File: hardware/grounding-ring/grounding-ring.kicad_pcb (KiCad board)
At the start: 2 copper layers, 28 x 38.2 mm, 1 part, among them P1 CONN_01X02

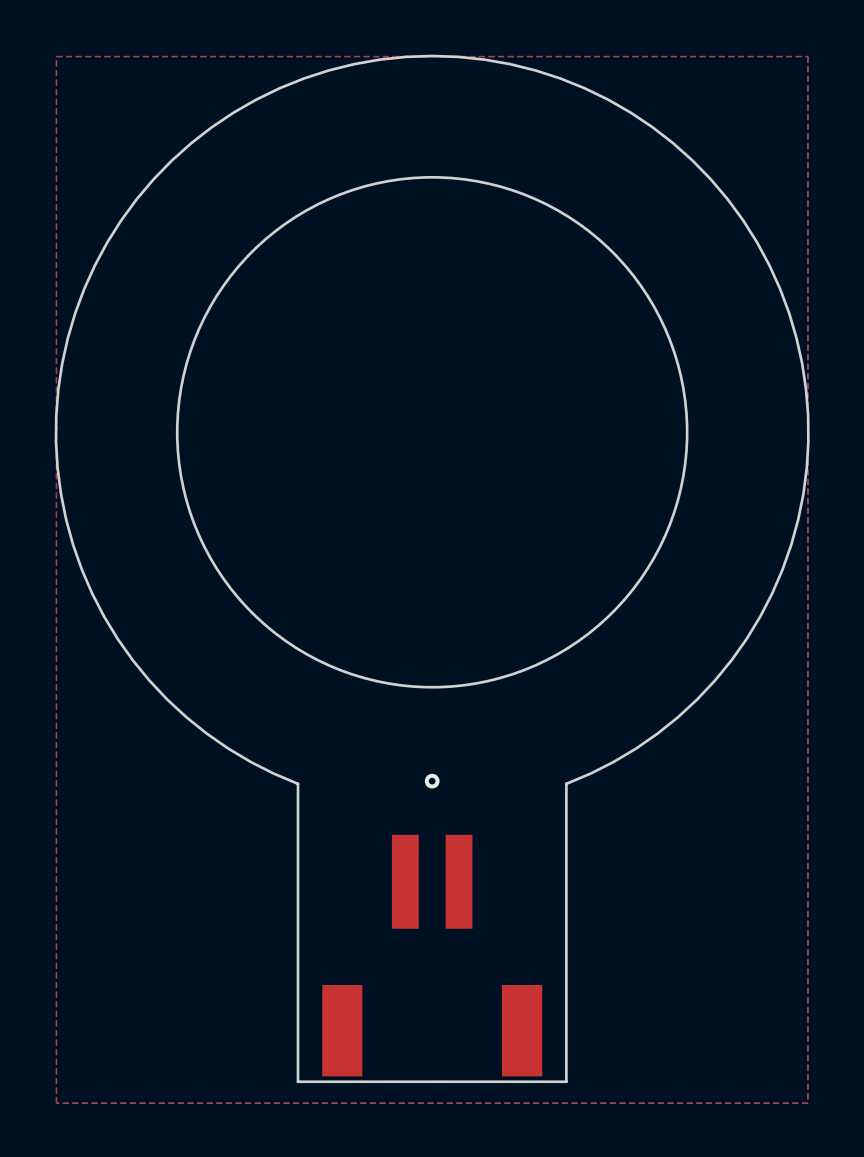
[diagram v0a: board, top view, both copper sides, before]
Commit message: grounding ring prototype
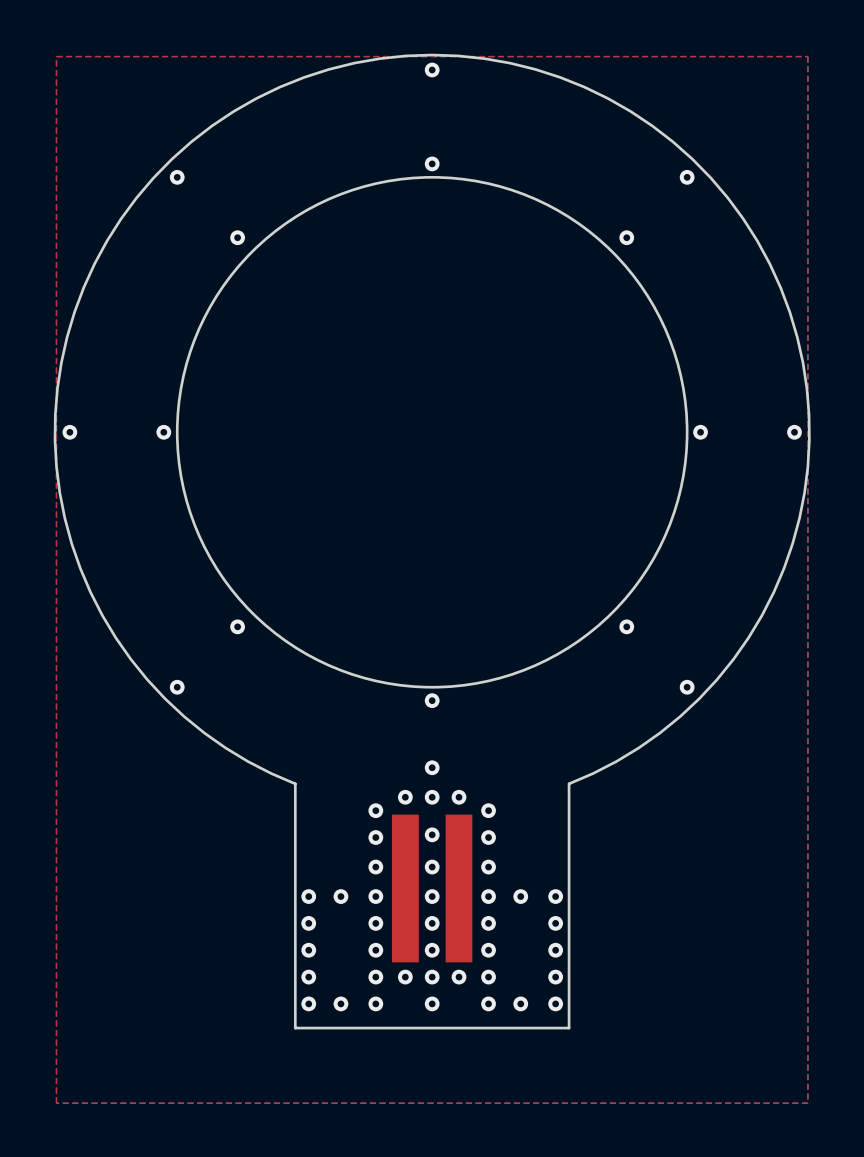
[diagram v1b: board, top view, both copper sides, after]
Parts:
- P1: footprint kicad-libraries:JST-PH-2 -> kicad-libraries:JST-PH-2-SMD
- moved P1 7.00 mm to (150.0, 117.0), turned to 180 degrees
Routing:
- net GND: vias 1 -> 58
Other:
- board size 28 x 38.2 mm -> 28.1 x 36.3 mm
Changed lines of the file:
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@@
     (thickness 1.6)
     (drawings 8)
-    (tracks 1)
+    (tracks 58)
     (zones 0)
     (modules 1)
@@
       (drillshape 0)
       (scaleselection 1)
-      (outputdirectory "../../../Schreibtisch/proto/breakout_V2/"))
+      (outputdirectory "../../../../Schreibtisch/proto/grounding-ring/"))
   )
   (net 0 "")
@@
     (add_net GND)
   )
-  (module kicad-libraries:JST-PH-2 (layer F.Cu)
-    (at 150 124)
-    (fp_text reference P1 (at 0 0) (layer F.Fab)
-      (effects (font (size 0.3 0.3) (thickness 0.075)))
+  (module kicad-libraries:JST-PH-2-SMD (layer F.Cu)
+    (at 150 117 180)
+    (fp_text reference P1 (at 0.09 -3.53) (layer F.Fab)
+      (effects (font (size 0.8 0.8) (thickness 0.15)))
     )
-    (fp_text value CONN_01X02 (at 0 0) (layer F.Fab)
-      (effects (font (size 0.3 0.3) (thickness 0.075)))
+    (fp_text value CONN_01X02 (at 0.48 -0.73) (layer F.Fab)
+      (effects (font (size 0.8 0.8) (thickness 0.15)))
     )
-    (fp_line (start -2.7 0) (end -2.1 -1.2) (layer F.Fab) (width 0.381))
-    (fp_line (start -2.1 -1.2) (end -1.6 0) (layer F.Fab) (width 0.381))
-    (fp_line (start 3.9 0) (end -3.9 0) (layer F.Fab) (width 0.381))
-    (fp_line (start -3.9 0) (end -3.9 -6) (layer F.Fab) (width 0.381))
-    (fp_line (start -3.9 -6) (end 3.9 -6) (layer F.Fab) (width 0.381))
-    (fp_line (start 3.9 -6) (end 3.9 0) (layer F.Fab) (width 0.381))
-    (pad 2 smd rect (at 1 -7.25) (size 1 3.5) (layers F.Cu F.Paste F.Mask)
+    (fp_line (start -3.975 -4.75) (end 3.975 -4.75) (layer F.Fab) (width 0.2))
+    (fp_line (start 3.975 -4.75) (end 3.975 0.25) (layer F.Fab) (width 0.2))
+    (fp_line (start 3.975 0.25) (end -3.975 0.25) (layer F.Fab) (width 0.2))
+    (fp_line (start -3.975 0.25) (end -3.975 -4.75) (layer F.Fab) (width 0.2))
+    (pad "" smd rect (at 3.4 -2.25 180) (size 1.6 3) (layers F.Paste F.Mask))
+    (pad "" smd rect (at -3.4 -2.25 180) (size 1.6 3) (layers F.Paste F.Mask))
+    (pad 2 smd rect (at 1 0 180) (size 1 5.5) (layers F.Cu F.Paste F.Mask)
       (net 1 GND))
-    (pad 1 smd rect (at -1 -7.25) (size 1 3.5) (layers F.Cu F.Paste F.Mask)
+    (pad 1 smd rect (at -1 0 180) (size 1 5.5) (layers F.Cu F.Paste F.Mask)
       (net 1 GND))
-    (pad EP smd rect (at 3.35 -1.7) (size 1.5 3.4) (layers F.Cu F.Paste F.Mask))
-    (pad EP smd rect (at -3.35 -1.7) (size 1.5 3.4) (layers F.Cu F.Paste F.Mask))
+    (model "../3d/Connectors/B2B-PH-SM4-TB(LF)(SN).wrl"
+      (at (xyz 0 0 0))
+      (scale (xyz 1 1 1))
+      (rotate (xyz 0 0 0))
+    )
   )
   (gr_poly (pts (xy 164 113) (xy 136 113) (xy 136 86) (xy 164 86)) (layer B.Mask) (width 0.1))
   (gr_poly (pts (xy 164 113) (xy 136 113) (xy 136 86) (xy 164 86)) (layer F.Mask) (width 0.1))
-  (gr_arc (start 150 100) (end 154.999999 113.099999) (angle -318.2183505) (layer Edge.Cuts) (width 0.1))
-  (gr_line (start 145 124.2) (end 145 113.1) (layer Edge.Cuts) (width 0.1))
-  (gr_line (start 155 124.2) (end 145 124.2) (layer Edge.Cuts) (width 0.1))
-  (gr_line (start 155 124.2) (end 155 113.1) (layer Edge.Cuts) (width 0.1))
+  (gr_arc (start 150 100) (end 155.1 113.099999) (angle -317.4567807) (layer Edge.Cuts) (width 0.1))
+  (gr_line (start 144.9 122.2) (end 144.9 113.1) (layer Edge.Cuts) (width 0.1))
+  (gr_line (start 155.1 122.2) (end 144.9 122.2) (layer Edge.Cuts) (width 0.1))
+  (gr_line (start 155.1 122.2) (end 155.1 113.1) (layer Edge.Cuts) (width 0.1))
   (gr_circle (center 150 100) (end 159.5 100) (layer Edge.Cuts) (width 0.1))
   (gr_text "Copyright Tinkerforge GmbH 2020.\nThis documentation describes Open Hardware and is licensed under the\nCERN OHL v. 1.1.\nYou may redistribute and modify this documentation under the terms of the\nCERN OHL v.1.1. (http://ohwr.org/cernohl). This documentation is distributed\nWITHOUT ANY EXPRESS OR IMPLIED WARRANTY, INCLUDING OF\nMERCHANTABILITY, SATISFACTORY QUALITY AND FITNESS FOR A\nPARTICULAR PURPOSE. Please see the CERN OHL v.1.1 for applicable\nconditions\n" (at 58.6 184.4) (layer F.Fab)
     (effects (font (size 1.5 1.5) (thickness 0.3)))
   )
-  (via (at 150 113) (size 0.55) (drill 0.25) (layers F.Cu B.Cu) (net 1))
+  (via (at 154.6 118.3) (size 0.55) (drill 0.25) (layers F.Cu B.Cu) (net 1))
+  (via (at 154.6 117.3) (size 0.55) (drill 0.25) (layers F.Cu B.Cu) (net 1))
+  (via (at 153.3 121.3) (size 0.55) (drill 0.25) (layers F.Cu B.Cu) (net 1))
+  (via (at 154.6 121.3) (size 0.55) (drill 0.25) (layers F.Cu B.Cu) (net 1))
+  (via (at 152.1 117.3) (size 0.55) (drill 0.25) (layers F.Cu B.Cu) (net 1))
+  (via (at 152.1 120.3) (size 0.55) (drill 0.25) (layers F.Cu B.Cu) (net 1))
+  (via (at 152.1 121.3) (size 0.55) (drill 0.25) (layers F.Cu B.Cu) (net 1))
+  (via (at 152.1 119.3) (size 0.55) (drill 0.25) (layers F.Cu B.Cu) (net 1))
+  (via (at 154.6 119.3) (size 0.55) (drill 0.25) (layers F.Cu B.Cu) (net 1))
+  (via (at 152.1 118.3) (size 0.55) (drill 0.25) (layers F.Cu B.Cu) (net 1))
+  (via (at 153.3 117.3) (size 0.55) (drill 0.25) (layers F.Cu B.Cu) (net 1))
+  (via (at 154.6 120.3) (size 0.55) (drill 0.25) (layers F.Cu B.Cu) (net 1))
+  (via (at 150 113.6) (size 0.55) (drill 0.25) (layers F.Cu B.Cu) (net 1))
+  (via (at 145.4 119.3) (size 0.55) (drill 0.25) (layers F.Cu B.Cu) (net 1))
+  (via (at 145.4 118.3) (size 0.55) (drill 0.25) (layers F.Cu B.Cu) (net 1))
+  (via (at 145.4 120.3) (size 0.55) (drill 0.25) (layers F.Cu B.Cu) (net 1))
+  (via (at 145.4 117.3) (size 0.55) (drill 0.25) (layers F.Cu B.Cu) (net 1))
+  (via (at 146.6 117.3) (size 0.55) (drill 0.25) (layers F.Cu B.Cu) (net 1))
+  (via (at 147.9 117.3) (size 0.55) (drill 0.25) (layers F.Cu B.Cu) (net 1))
+  (via (at 147.9 118.3) (size 0.55) (drill 0.25) (layers F.Cu B.Cu) (net 1))
+  (via (at 147.9 119.3) (size 0.55) (drill 0.25) (layers F.Cu B.Cu) (net 1))
+  (via (at 147.9 120.3) (size 0.55) (drill 0.25) (layers F.Cu B.Cu) (net 1))
+  (via (at 147.9 121.3) (size 0.55) (drill 0.25) (layers F.Cu B.Cu) (net 1))
+  (via (at 146.6 121.3) (size 0.55) (drill 0.25) (layers F.Cu B.Cu) (net 1))
+  (via (at 145.4 121.3) (size 0.55) (drill 0.25) (layers F.Cu B.Cu) (net 1))
+  (via (at 150 115) (size 0.55) (drill 0.25) (layers F.Cu B.Cu) (net 1))
+  (via (at 150 116.2) (size 0.55) (drill 0.25) (layers F.Cu B.Cu) (net 1))
+  (via (at 150 117.3) (size 0.55) (drill 0.25) (layers F.Cu B.Cu) (net 1))
+  (via (at 150 118.3) (size 0.55) (drill 0.25) (layers F.Cu B.Cu) (net 1))
+  (via (at 150 119.3) (size 0.55) (drill 0.25) (layers F.Cu B.Cu) (net 1))
+  (via (at 150 120.3) (size 0.55) (drill 0.25) (layers F.Cu B.Cu) (net 1))
+  (via (at 150 121.3) (size 0.55) (drill 0.25) (layers F.Cu B.Cu) (net 1))
+  (via (at 149 120.3) (size 0.55) (drill 0.25) (layers F.Cu B.Cu) (net 1))
+  (via (at 151 120.3) (size 0.55) (drill 0.25) (layers F.Cu B.Cu) (net 1))
+  (via (at 149 113.6) (size 0.55) (drill 0.25) (layers F.Cu B.Cu) (net 1))
+  (via (at 151 113.6) (size 0.55) (drill 0.25) (layers F.Cu B.Cu) (net 1))
+  (via (at 152.1 116.2) (size 0.55) (drill 0.25) (layers F.Cu B.Cu) (net 1))
+  (via (at 152.1 115.1) (size 0.55) (drill 0.25) (layers F.Cu B.Cu) (net 1))
+  (via (at 152.1 114.1) (size 0.55) (drill 0.25) (layers F.Cu B.Cu) (net 1))
+  (via (at 147.9 114.1) (size 0.55) (drill 0.25) (layers F.Cu B.Cu) (net 1))
+  (via (at 147.9 116.2) (size 0.55) (drill 0.25) (layers F.Cu B.Cu) (net 1))
+  (via (at 147.9 115.1) (size 0.55) (drill 0.25) (layers F.Cu B.Cu) (net 1))
+  (via (at 136.5 100) (size 0.55) (drill 0.25) (layers F.Cu B.Cu) (net 1))
+  (via (at 140 100) (size 0.55) (drill 0.25) (layers F.Cu B.Cu) (net 1))
+  (via (at 160 100) (size 0.55) (drill 0.25) (layers F.Cu B.Cu) (net 1))
+  (via (at 163.5 100) (size 0.55) (drill 0.25) (layers F.Cu B.Cu) (net 1))
+  (via (at 150 90) (size 0.55) (drill 0.25) (layers F.Cu B.Cu) (net 1))
+  (via (at 150 86.5) (size 0.55) (drill 0.25) (layers F.Cu B.Cu) (net 1))
+  (via (at 150 110) (size 0.55) (drill 0.25) (layers F.Cu B.Cu) (net 1))
+  (via (at 150 112.5) (size 0.55) (drill 0.25) (layers F.Cu B.Cu) (net 1))
+  (via (at 142.75 107.25) (size 0.55) (drill 0.25) (layers F.Cu B.Cu) (net 1))
+  (via (at 140.5 109.5) (size 0.55) (drill 0.25) (layers F.Cu B.Cu) (net 1))
+  (via (at 157.25 107.25) (size 0.55) (drill 0.25) (layers F.Cu B.Cu) (net 1))
+  (via (at 159.5 109.5) (size 0.55) (drill 0.25) (layers F.Cu B.Cu) (net 1))
+  (via (at 142.75 92.75) (size 0.55) (drill 0.25) (layers F.Cu B.Cu) (net 1))
+  (via (at 140.5 90.5) (size 0.55) (drill 0.25) (layers F.Cu B.Cu) (net 1))
+  (via (at 157.25 92.75) (size 0.55) (drill 0.25) (layers F.Cu B.Cu) (net 1))
+  (via (at 159.5 90.5) (size 0.55) (drill 0.25) (layers F.Cu B.Cu) (net 1))
   (zone (net 1) (net_name GND) (layer F.Cu) (hatch edge 0.508)
-    (connect_pads (clearance 0.2))
+    (connect_pads yes (clearance 0.2))
     (min_thickness 0.254)
     (fill yes (arc_segments 32) (thermal_gap 0.508) (thermal_bridge_width 0.508))
